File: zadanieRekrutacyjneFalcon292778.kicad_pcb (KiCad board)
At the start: 2 copper layers, 65 parts, among them J1 Conn_01x03_Pin, J2 Conn_01x02_Pin, J3 Conn_01x02_Pin, J4 Conn_01x04_Pin, J5 Conn_01x08_Pin, J6 Conn_01x08_Pin, J7 Conn_01x02_Pin, SW1 CK_KMS2xxG, SW2 SW_Nidec_CAS-120A1, SW3 CK_KMS2xxG, SW4 CK_KMS2xxG, SW5 SW_Nidec_CAS-120A1, U1 ESP32-S3, U2 AMS1117, U3 BMI270, U4 W25Q128JVE, U5 ESPSRAM, Y1 Crystal

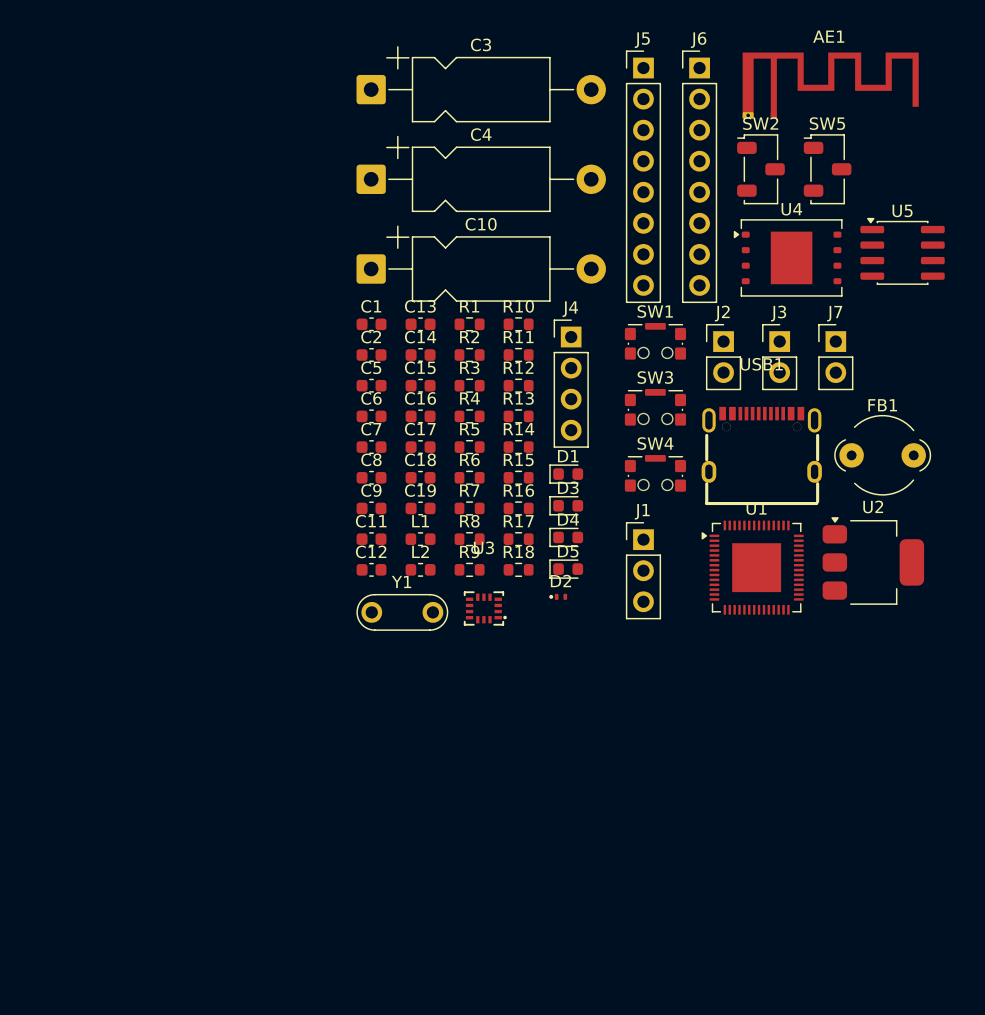
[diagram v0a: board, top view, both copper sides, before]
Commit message: placement + testowy tracking v1
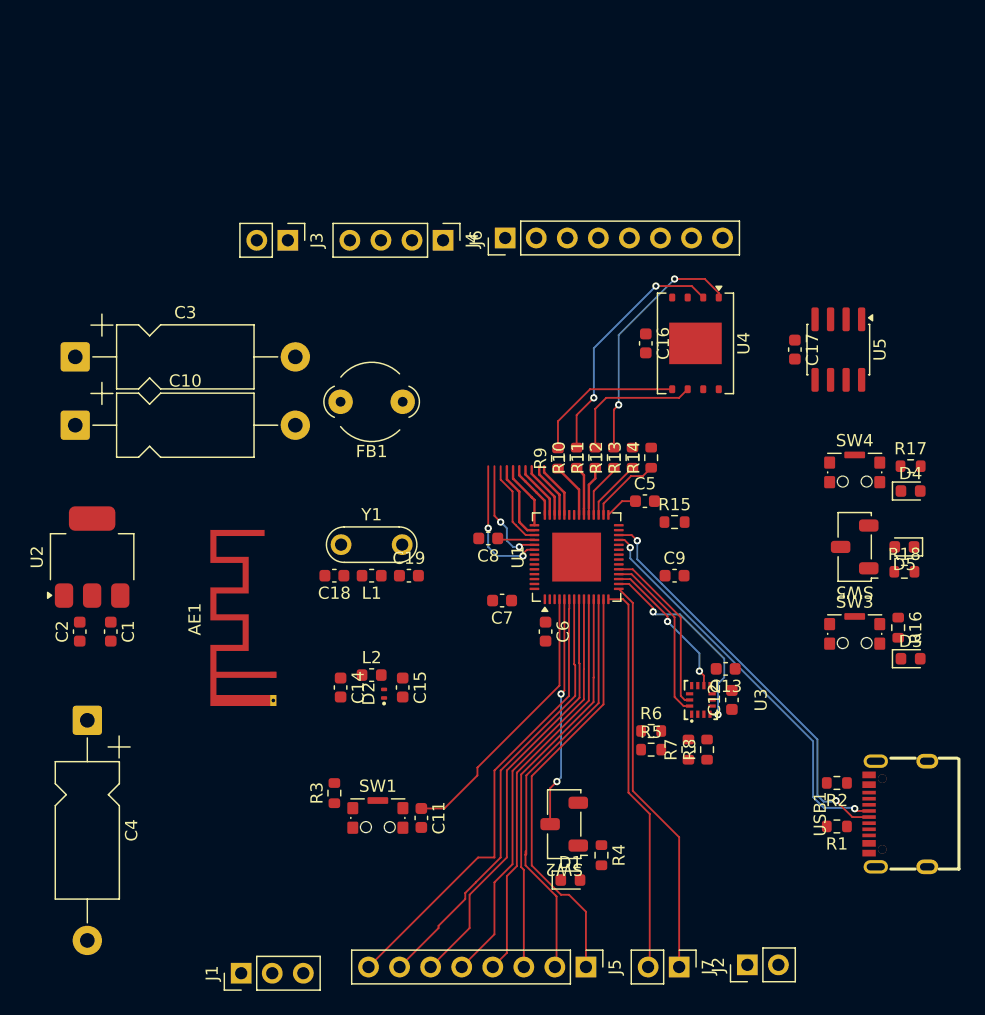
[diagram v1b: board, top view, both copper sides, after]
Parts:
- moved J5 73.7 mm to (159.4, 117.7), turned to -90 degrees
- moved U2 63.9 mm to (119.0, 84.1), turned to 90 degrees
- moved AE1 61.4 mm to (133.8, 93.8), turned to 90 degrees
- moved SW2 55.9 mm to (157.6, 106.0), turned to 180 degrees
- moved J7 52.7 mm to (167.0, 117.7), turned to -90 degrees
- moved J2 51.0 mm to (172.6, 117.5), turned to 90 degrees
- moved R1 50.9 mm to (179.9, 106.2), turned to 180 degrees
- moved C4 50.0 mm to (118.6, 97.5), turned to -90 degrees
- moved J1 48.4 mm to (131.2, 118.2), turned to 90 degrees
- moved R2 46.1 mm to (179.9, 102.6), turned to 180 degrees
- moved SW1 44.9 mm to (142.4, 105.5)
- moved J3 41.1 mm to (135.0, 58.2), turned to -90 degrees
- moved C13 37.6 mm to (170.8, 93.3), turned to 180 degrees
- moved R4 37.5 mm to (160.6, 108.5), turned to -90 degrees
- moved FB1 37.0 mm to (144.4, 71.4), turned to 180 degrees
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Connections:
- J4 pad 1: /JTAGMS -> /JTAGI
- J4 pad 4: /JTAGI -> /JTAGMS
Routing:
- net /BAJT1-0: track 0.00 -> 37.7 mm
- net /BAJT1-1: track 0.00 -> 36.1 mm
- net /BAJT1-2: track 0.00 -> 35.1 mm
- net /BAJT1-7: track 0.00 -> 34.7 mm
- net /BAJT1-3: track 0.00 -> 34.2 mm
- net /BAJT1-6: track 0.00 -> 34.0 mm
- net /USB+: track 0.00 -> 33.6 mm, vias 0 -> 2
- net /BAJT1-4: track 0.00 -> 33.3 mm
- net /USB-: track 0.00 -> 33.0 mm, vias 0 -> 2
- net /GPIO2: track 0.00 -> 33.0 mm
- net /BAJT1-5: track 0.00 -> 32.6 mm
- net /GPIO1: track 0.00 -> 32.3 mm
- net Net-(U1-CHIP_PU): track 0.00 -> 22.9 mm
- net /FLASH: track 0.00 -> 20.3 mm, vias 0 -> 2
- net /SPI1: track 0.00 -> 20.2 mm, vias 0 -> 2
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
